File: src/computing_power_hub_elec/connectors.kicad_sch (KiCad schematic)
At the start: 49 parts, among them J105 BM03B-PASS, J106 BM03B-PASS, J107 BM03B-PASS, J108 BM03B-PASS, J310 XT30M, J320 RJ45, J321 RJ45, J330 S2P-VH, J340 S2P-VH, Q301 BC846S,115, Q340 SSM3K333R, Q350 SSM3K333R

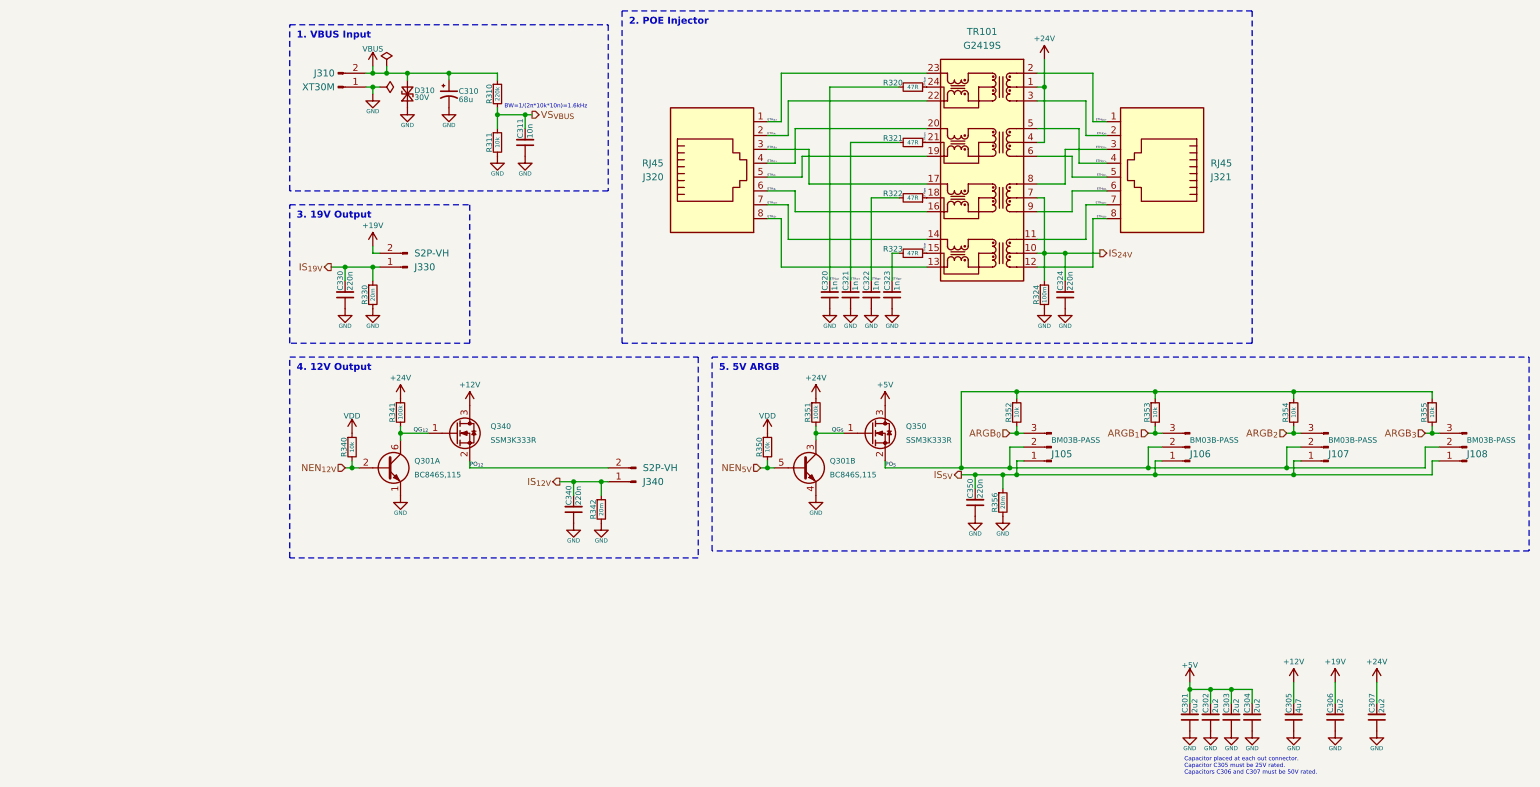
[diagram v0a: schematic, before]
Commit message: Baa
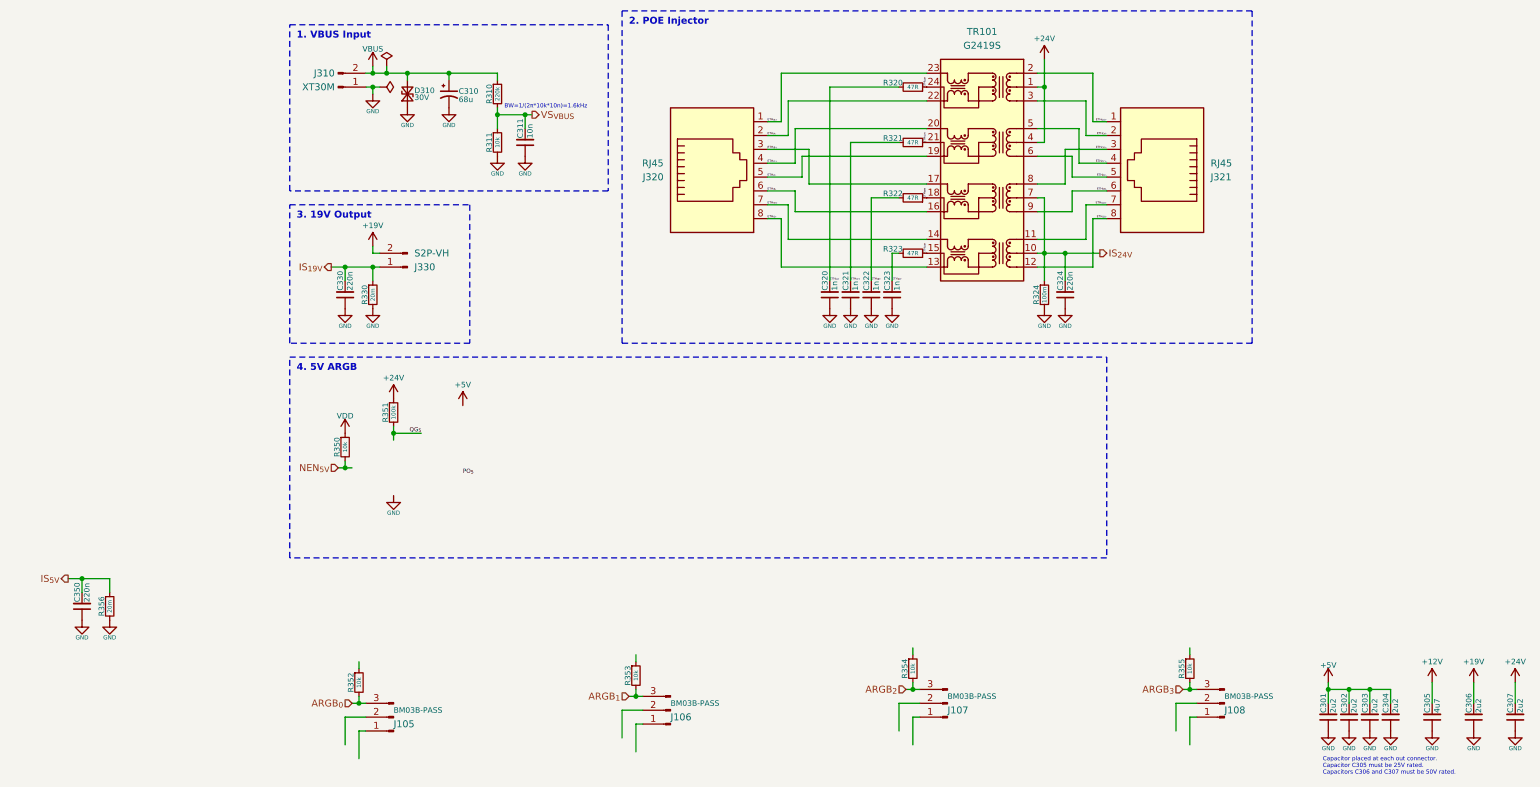
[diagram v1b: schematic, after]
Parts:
- removed C340: 220n, Capacitor_SMD:C_0402_1005Metric, symbol Bluesat:C_CompactV
- removed J340: S2P-VH, symbol Connector:Conn_01x02_Pin
- removed Q301: BC846S,115, Package_TO_SOT_SMD:SOT-363_SC-70-6, symbol Transistor_BJT:Q_Dual_NPN_NPN_E1B1C2E2B2C1
- removed Q340, Q350: SSM3K333R, Package_TO_SOT_SMD:SOT-23, symbol Transistor_FET:Q_NMOS_GSD
- removed R340: 10k, Resistor_SMD:R_0402_1005Metric, symbol Bluesat:R_CompactV
- removed R341: 100k, Resistor_SMD:R_0402_1005Metric, symbol Bluesat:R_CompactV
- removed R342: 20m, Diode_SMD:D_2512_6332Metric, symbol Bluesat:R_CompactV
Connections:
- net IS_{5V}: no longer J105.1 (Pin_1), J106.1 (Pin_1), J107.1 (Pin_1), J108.1 (Pin_1)
- net PO_{5}: no longer J105.2 (Pin_2), J106.2 (Pin_2), J107.2 (Pin_2), J108.2 (Pin_2), R352.1, R353.1, R354.1, R355.1
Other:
- note added: "4. 5V ARGB"
- note removed: "4. 12V Output"
- note removed: "5. 5V ARGB"
- moved on the sheet: C301, C302, C303, C304, C305, C306, C307, C350, J105, J106, J107, J108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
